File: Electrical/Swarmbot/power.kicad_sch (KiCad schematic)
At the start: 39 parts, among them J3 Charging Header, J4 Battery 1S2P, SW3 SW_SPST, U6 TP4056, U7 FP6298, U8 AP9101CK, U9 AP2112K-3.3

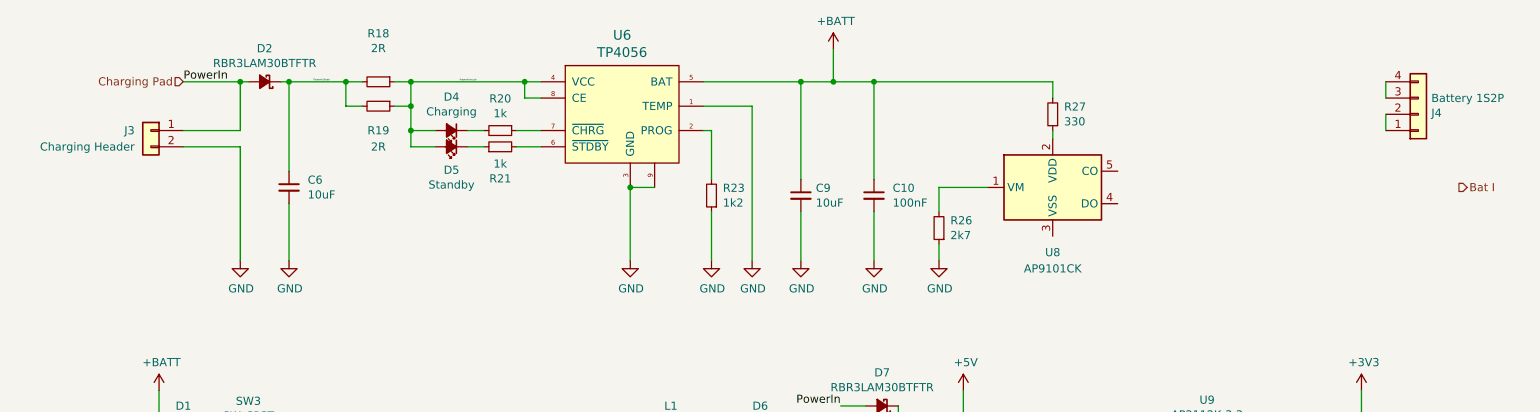
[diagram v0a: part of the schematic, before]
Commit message: some little changes have been made
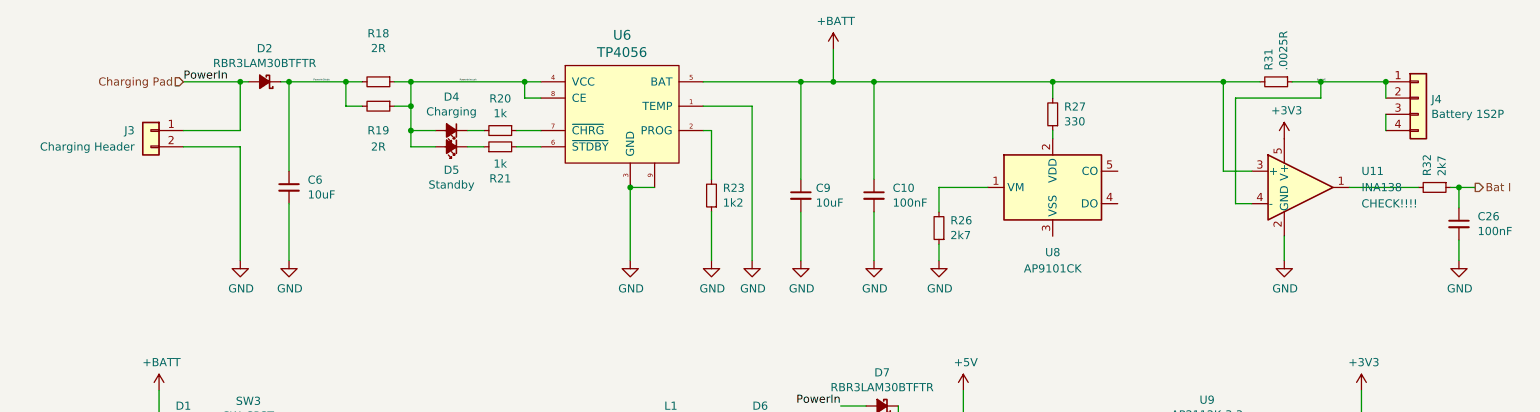
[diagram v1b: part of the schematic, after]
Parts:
- added C26: 100nF, Capacitor_SMD:C_0805_2012Metric_Pad1.18x1.45mm_HandSolder, symbol Device:C_Small
- added R31: .0025R, Resistor_SMD:R_1206_3216Metric_Pad1.30x1.75mm_HandSolder, symbol Device:R_Small
- added R32: 2k7, Resistor_SMD:R_0805_2012Metric_Pad1.20x1.40mm_HandSolder, symbol Device:R_Small
- added U11: INA138, Package_TO_SOT_SMD:SOT-23-5, symbol Amplifier_Current:INA138
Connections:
- net PowerIn is gone; now on net Charging Pad: D2.2 (A), D7.2 (A), J3.1 (Pin_1)
- net +3V3: now also U11.5 (V+)
- net +BATT: now also R31.2, U11.3 (+)
- net Bat I: now also C26.1, R32.1
- net GND: now also C26.2, U11.2 (GND)
- net Bat+VE: now reaches J4.1 (Pin_1), J4.2 (Pin_2)
- net Bat+VE: now also R31.1, U11.4 (-)
- new net: R32.2, U11.1
